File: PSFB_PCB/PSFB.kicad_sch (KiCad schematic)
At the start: 54 parts, among them IC10 ISOUSB111DWXR, J10 V_IN_SENSE, J11 I_OUT_SENSE, J12 V_OUT_SENSE, J13 V_BAT_SENSE, J14 GND_SENSE, J15 CTRL_AH, J16 CTRL_AL, J17 CTRL_BL, J18 CTRL_BH, J2 GND_S, J20 5VCC_S, J21 Vref_S, J22 VDC_S_SENSE_S, J3 JUMPER_BOOT, J5 STLINK_PIN, J6 USB_C, J9 I_IN_SENSE, T1 MAIN TRANSFORMER, U1 STM32G474CBTx

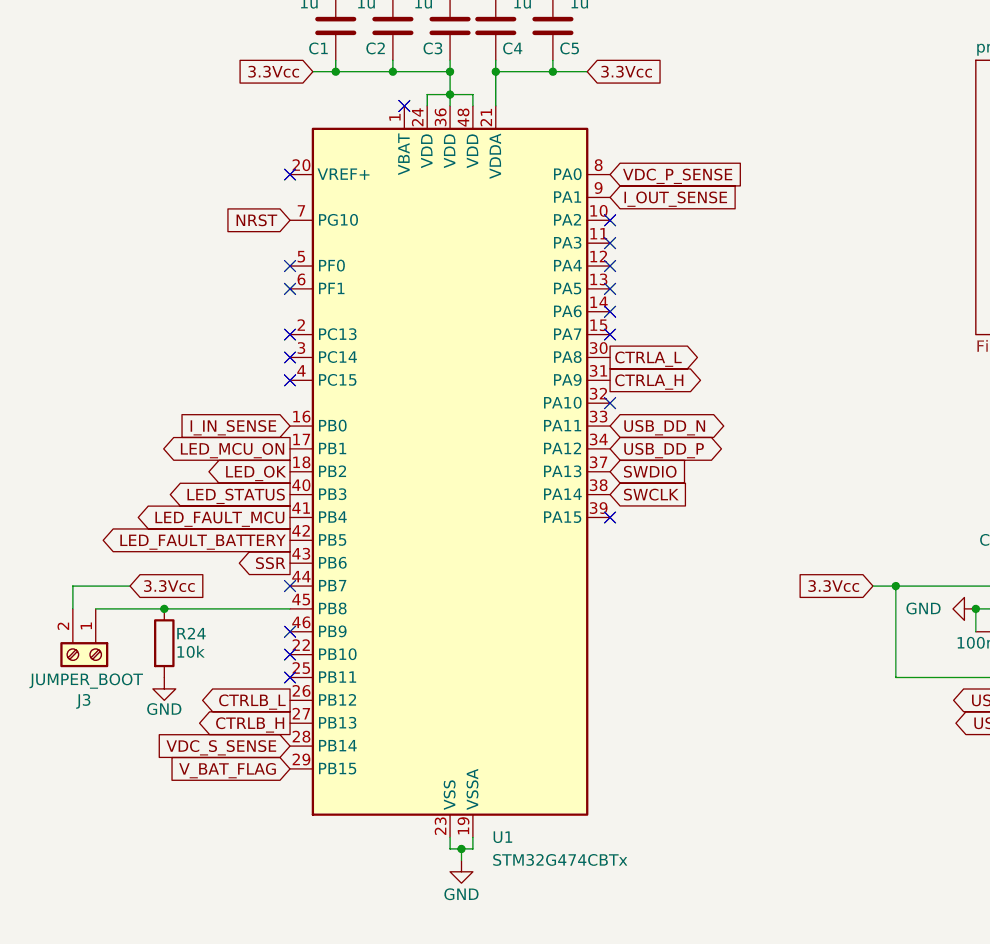
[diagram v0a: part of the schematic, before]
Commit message: MCU conections
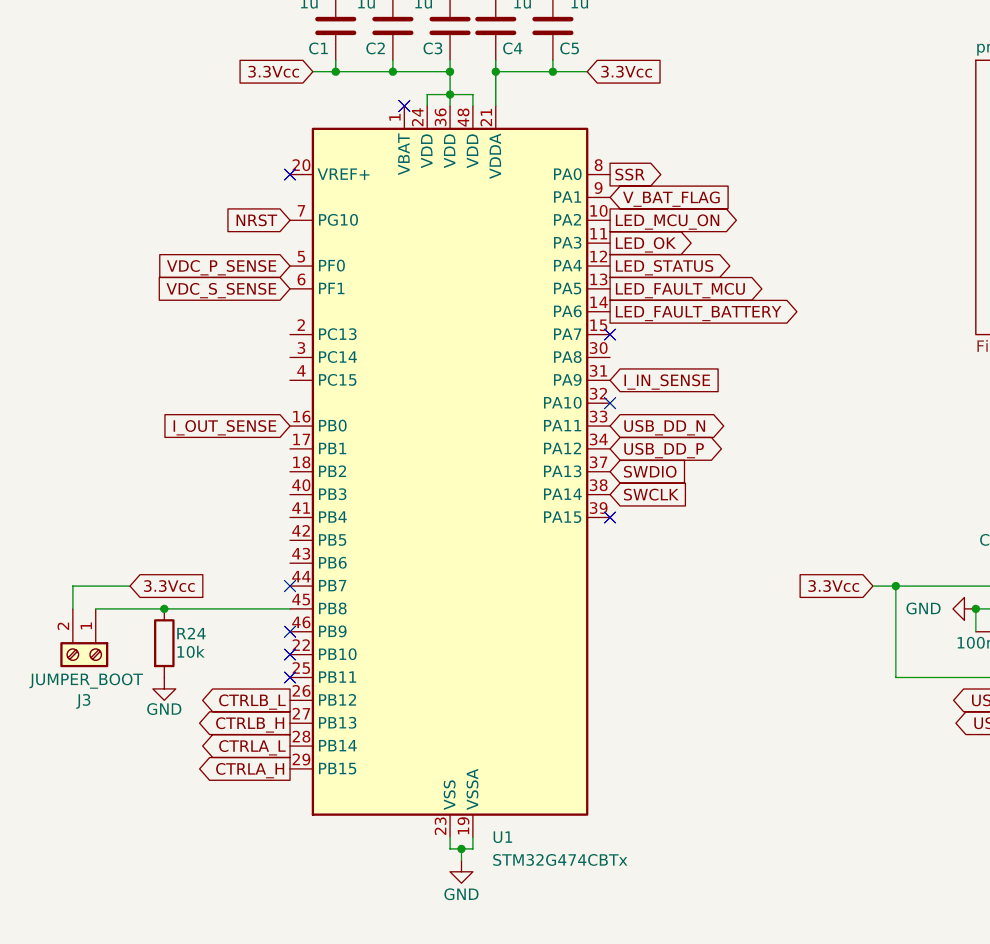
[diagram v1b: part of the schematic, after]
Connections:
- net CTRLA_H: now also U1.29 (PB15); no longer U1.31 (PA9)
- net CTRLA_L: now also U1.28 (PB14); no longer U1.30 (PA8)
- net I_IN_SENSE: now also U1.31 (PA9); no longer U1.16 (PB0)
- net I_OUT_SENSE: now also U1.16 (PB0); no longer U1.9 (PA1)
- net LED_FAULT_BATTERY: now also U1.14 (PA6); no longer U1.42 (PB5)
- net LED_FAULT_MCU: now also U1.13 (PA5); no longer U1.41 (PB4)
- net LED_MCU_ON: now also U1.10 (PA2); no longer U1.17 (PB1)
- net LED_OK: now also U1.11 (PA3); no longer U1.18 (PB2)
- net LED_STATUS: now also U1.12 (PA4); no longer U1.40 (PB3)
- net SSR: now also U1.8 (PA0); no longer U1.43 (PB6)
- net VDC_P_SENSE: now also U1.5 (PF0); no longer U1.8 (PA0)
- net VDC_S_SENSE: now also U1.6 (PF1); no longer U1.28 (PB14)
- net V_BAT_FLAG: now also U1.9 (PA1); no longer U1.29 (PB15)
- no-connect marks 24 -> 14
